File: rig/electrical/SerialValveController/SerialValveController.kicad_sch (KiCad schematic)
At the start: 21 parts, among them J1 Screw_Terminal_01x02, J17 Conn_01x05_Socket, J18 TST-105-01-X-D, J19 TST-105-01-X-D, J2 Screw_Terminal_01x02, U1 TPIC6595

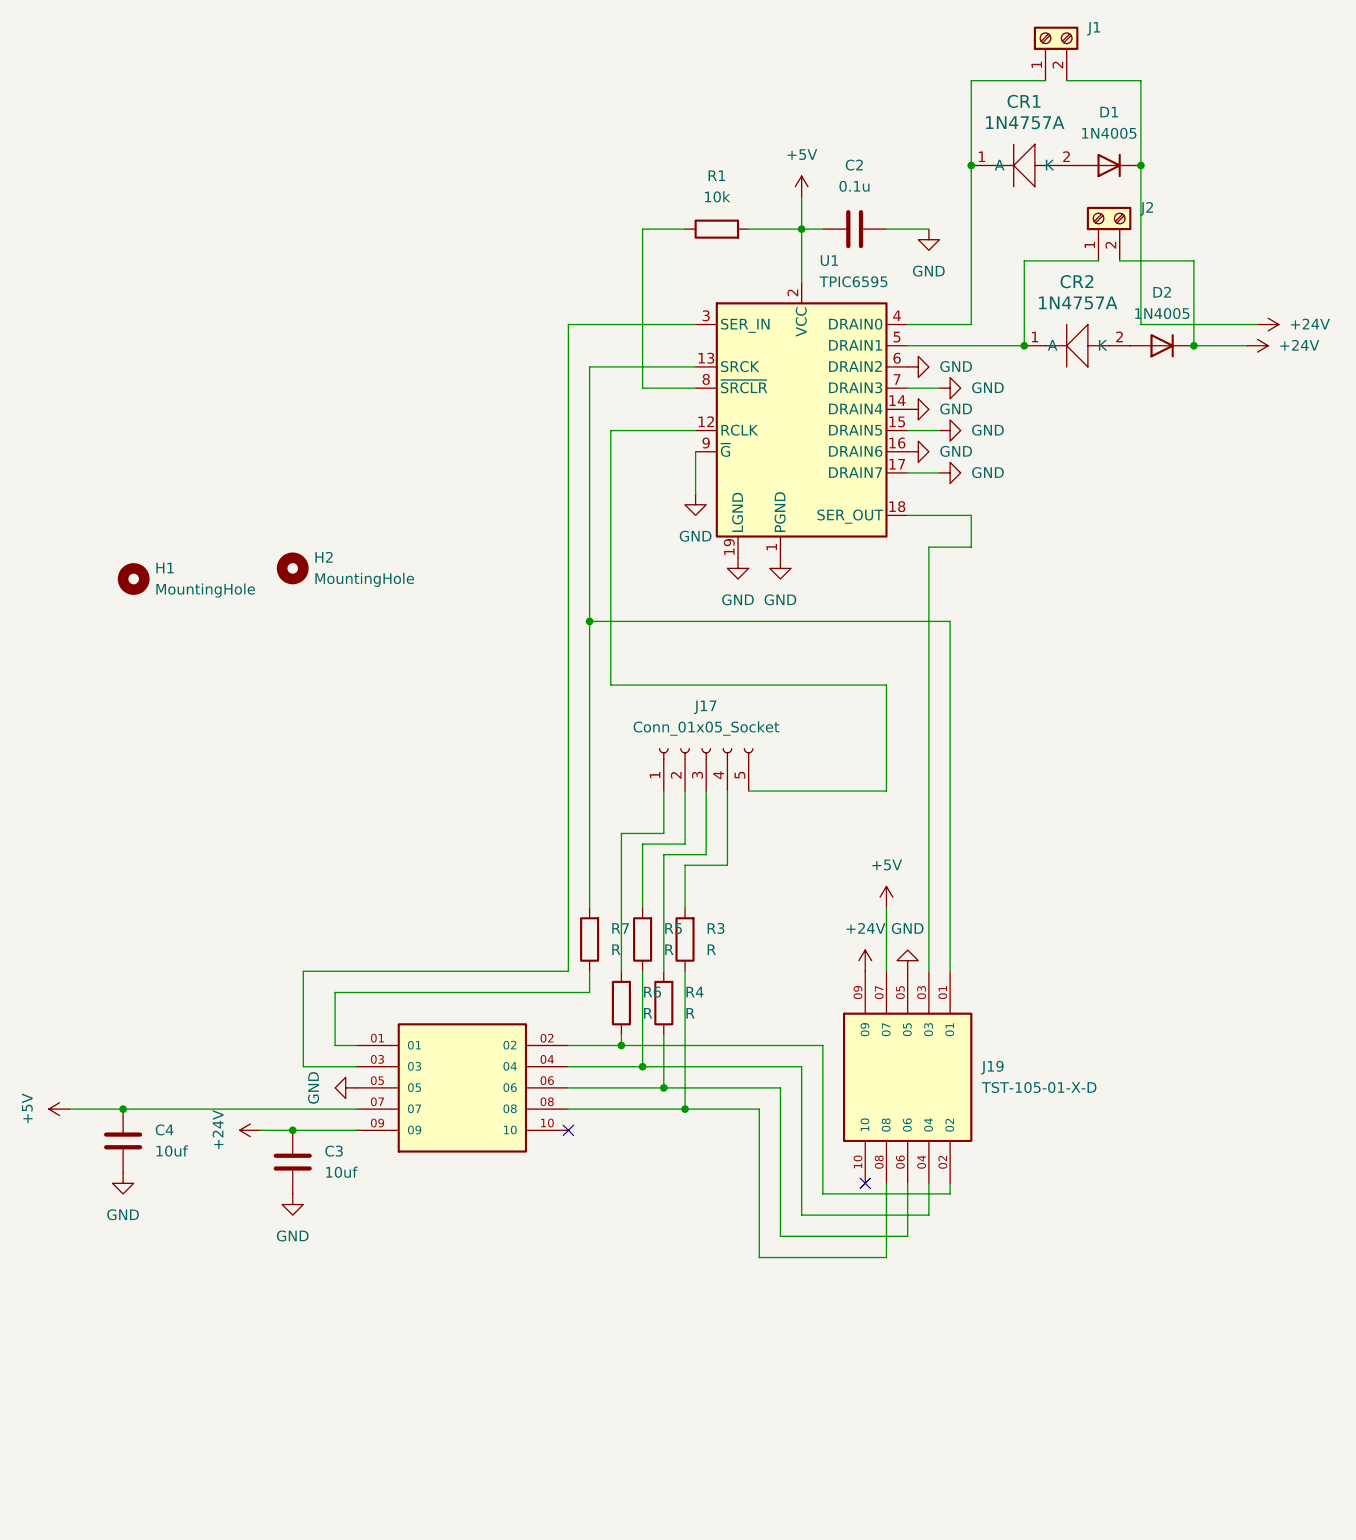
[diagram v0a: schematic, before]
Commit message: Serial Olfactometer improved design
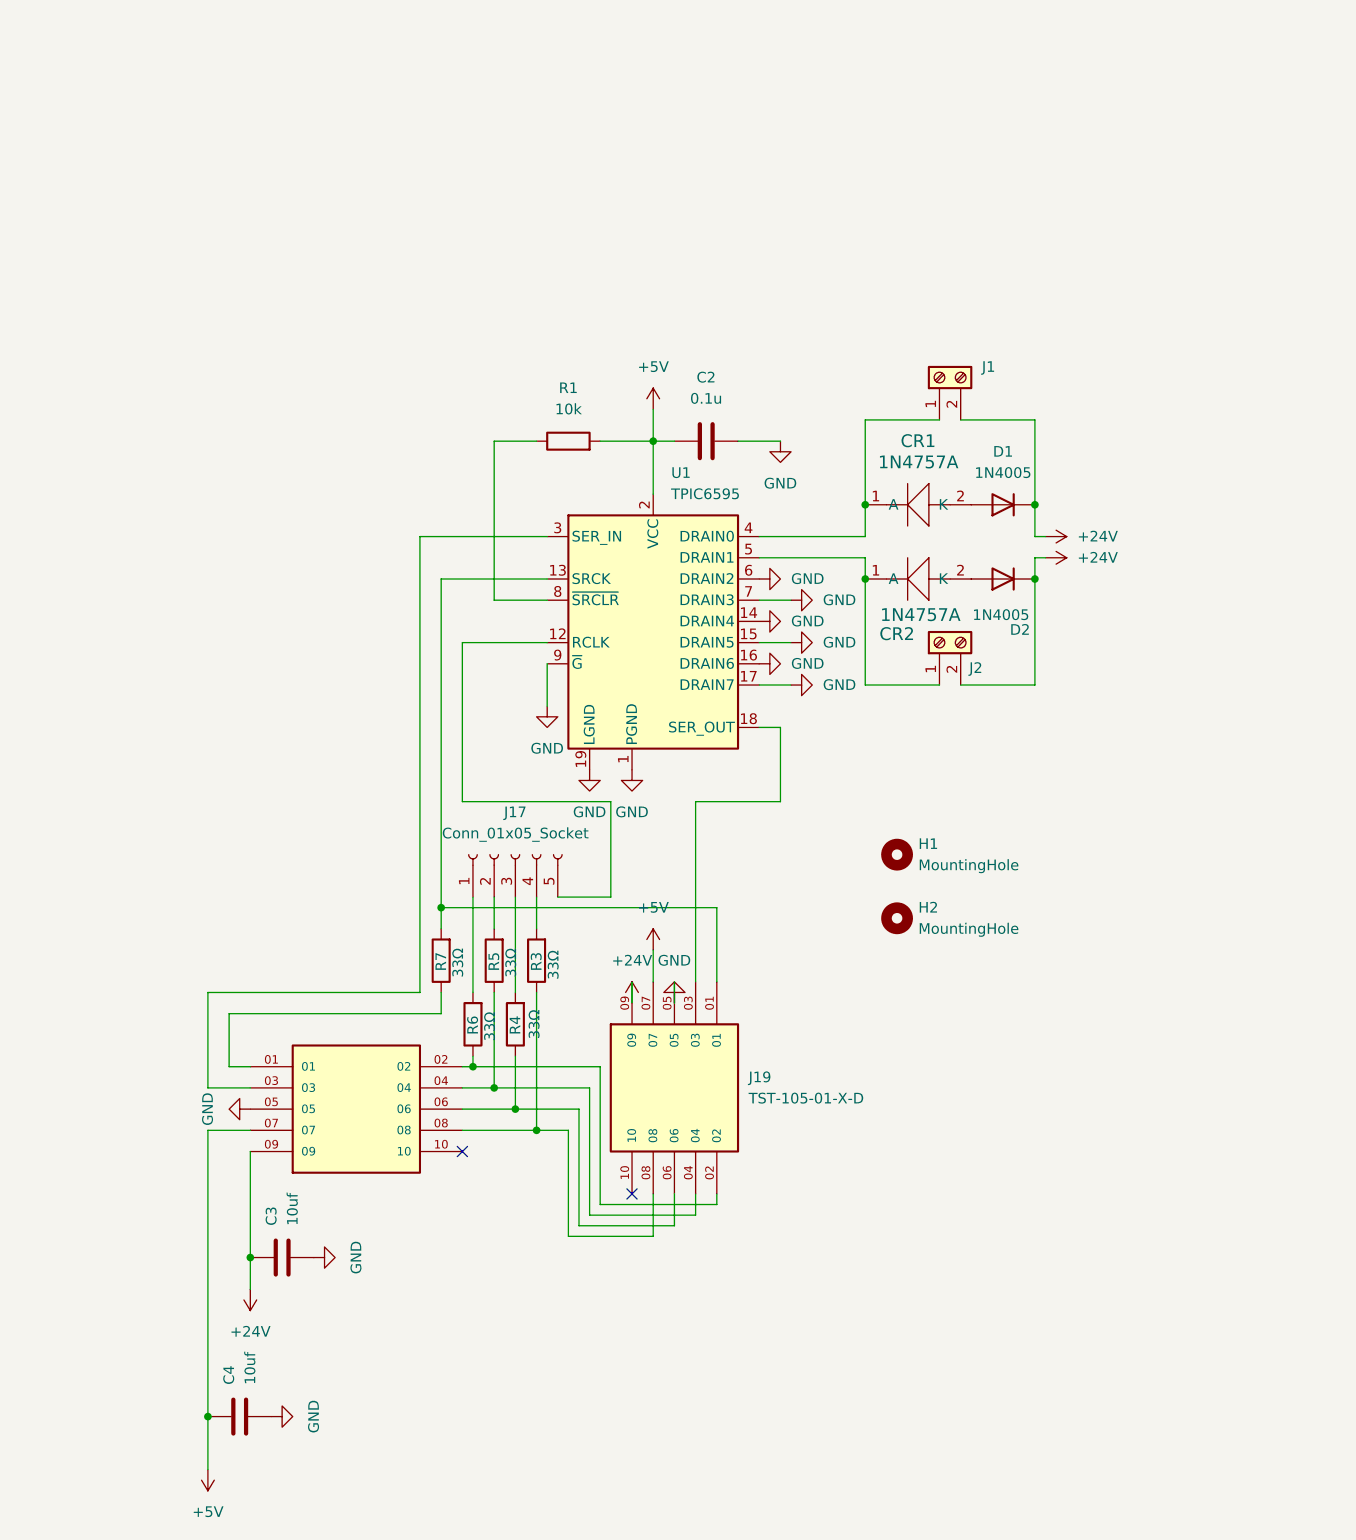
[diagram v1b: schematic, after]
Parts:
- R3, R4, R5, R6, R7: value R -> 33Ω
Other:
- company: (none) -> Ruta and Kronauer Labs, Rockefeller University
- title: (none) -> MultiBiOS Serial Valve Controller
- moved on the sheet: C2, C3, C4, CR1, CR2, D1, D2, H1, H2, J1, J17, J19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
